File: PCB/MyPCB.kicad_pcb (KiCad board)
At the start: 2 copper layers, 82.4 x 43.4 mm, 10 parts, among them J1 OLED_DISPLAY, SW1 SW_Push, SW2 SW_Push, SW3 SW_Push, SW4 SW_Push, U1 XIAO-RP2040-DIP

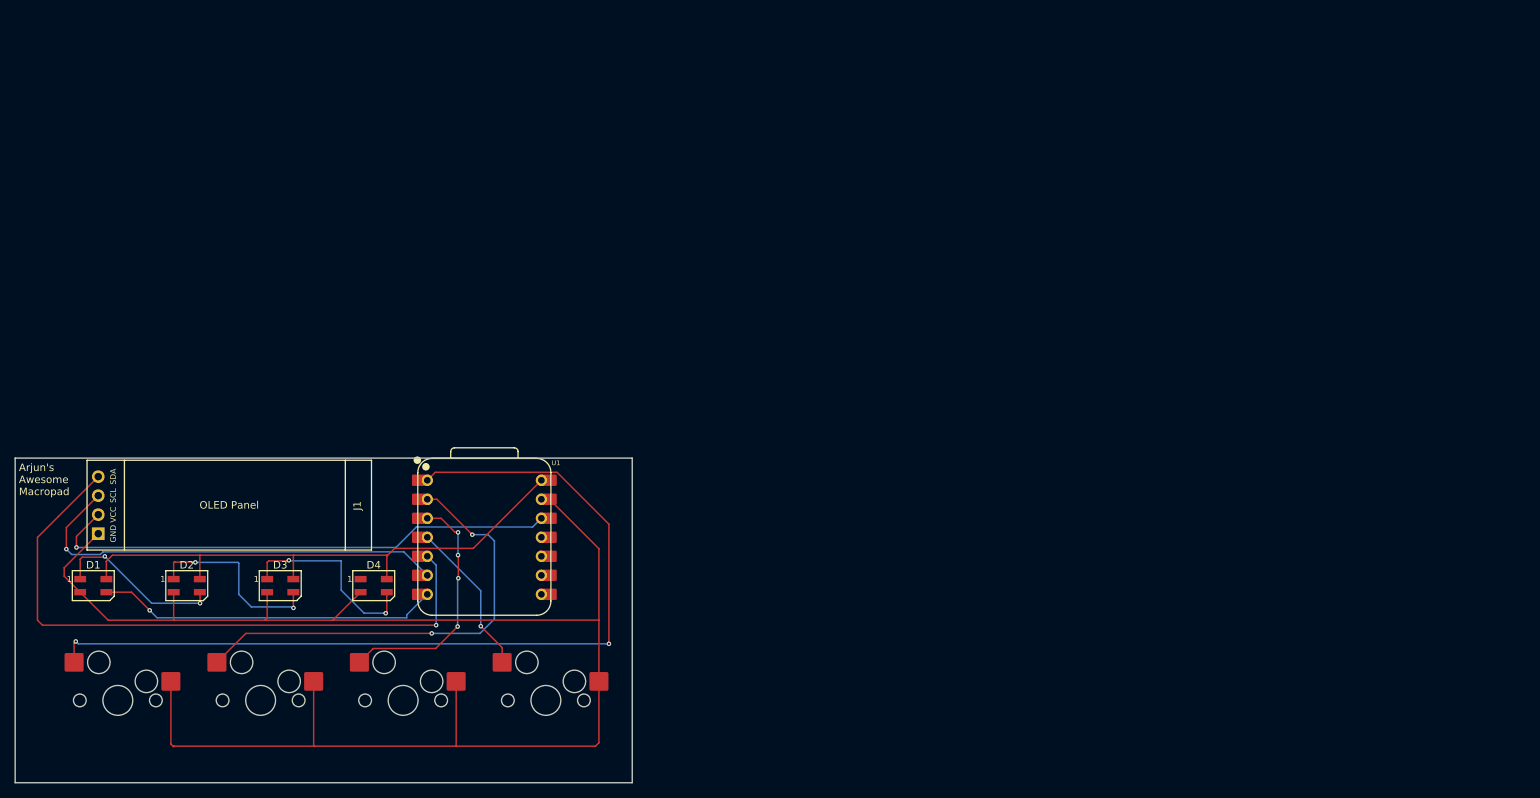
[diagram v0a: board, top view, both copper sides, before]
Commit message: finish case
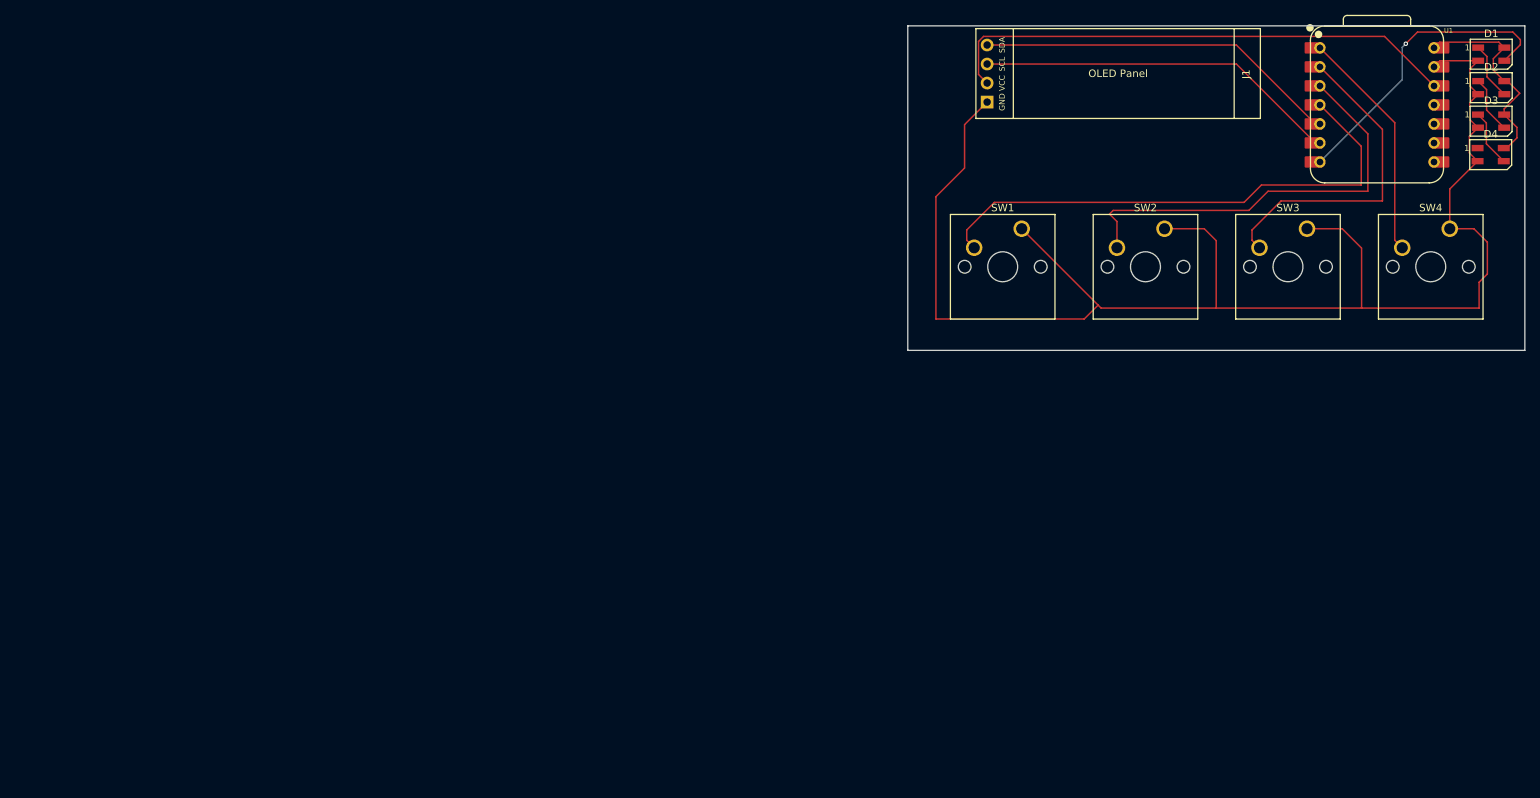
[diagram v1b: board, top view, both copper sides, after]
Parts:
- SW1, SW2, SW3, SW4: footprint MXCHERRY:MX-Hotswap-1U -> Button_Switch_Keyboard:SW_Cherry_MX_1.00u_PCB
- moved D1 199.8 mm to (237.1, 87.2)
- moved D2 186.5 mm to (237.1, 91.6)
- moved D3 173.2 mm to (237.1, 96.1)
- moved D4 159.9 mm to (237.1, 100.6)
- moved SW2 136.2 mm to (193.5, 110.5)
- moved SW1 136.2 mm to (174.4, 110.5)
- moved SW3 136.2 mm to (212.5, 110.5)
- moved SW4 136.2 mm to (231.6, 110.5)
- moved U1 132.5 mm to (221.9, 94.0)
- moved J1 132.0 mm to (206.3, 95.8)
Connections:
- SW1 pad 2: Net-(U1-GPIO26/ADC0/A0) -> Net-(U1-GPIO29/ADC3/A3)
- SW2 pad 2: Net-(U1-GPIO27/ADC1/A1) -> Net-(U1-GPIO28/ADC2/A2)
- SW3 pad 2: Net-(U1-GPIO28/ADC2/A2) -> Net-(U1-GPIO27/ADC1/A1)
- SW4 pad 2: Net-(U1-GPIO29/ADC3/A3) -> Net-(U1-GPIO26/ADC0/A0)
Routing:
- net Net-(U1-GPIO26/ADC0/A0): track 117.8 -> 31.3 mm, vias 2 -> 0
- net Net-(U1-GPIO29/ADC3/A3): track 20.8 -> 71.0 mm, vias 1 -> 0
- net +5V: track 74.7 -> 28.3 mm
- net SDA: track 85.8 -> 48.8 mm, vias 1 -> 0
- net Net-(U1-GPIO28/ADC2/A2): track 32.6 -> 57.4 mm, vias 4 -> 0
- net Net-(D3-DOUT): track 26.3 -> 7.65 mm, vias 2 -> 0
- net Net-(D2-DOUT): track 25.7 -> 7.66 mm, vias 2 -> 0
- net Net-(U1-GPIO27/ADC1/A1): track 61.2 -> 43.2 mm, vias 2 -> 0
- net Net-(D1-DOUT): track 22.9 -> 7.67 mm, vias 2 -> 0
- net GND: track 214.7 -> 202.6 mm
- net SCL: track 58.9 -> 48.8 mm, vias 1 -> 0
- net Net-(D1-DIN): track 46.0 -> 40.6 mm
- net 3V3: track 69.3 -> 69.9 mm, vias 1 -> 0
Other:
- board size 82.4 x 43.4 mm -> 82.4 x 43.3 mm
